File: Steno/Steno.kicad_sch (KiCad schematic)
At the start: 25 parts

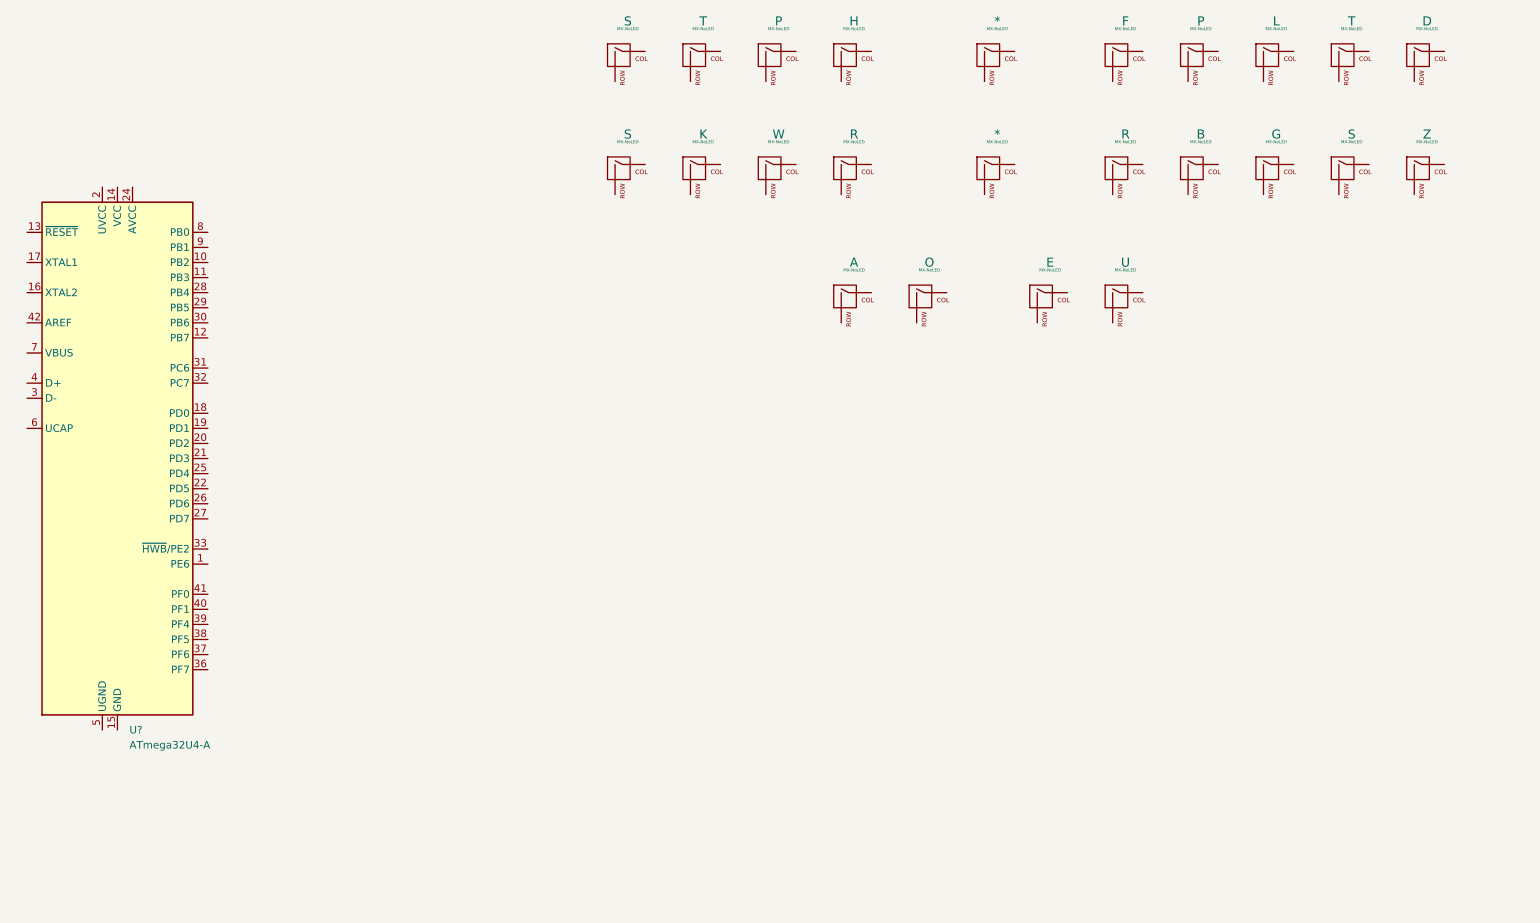
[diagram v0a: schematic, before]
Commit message: asd
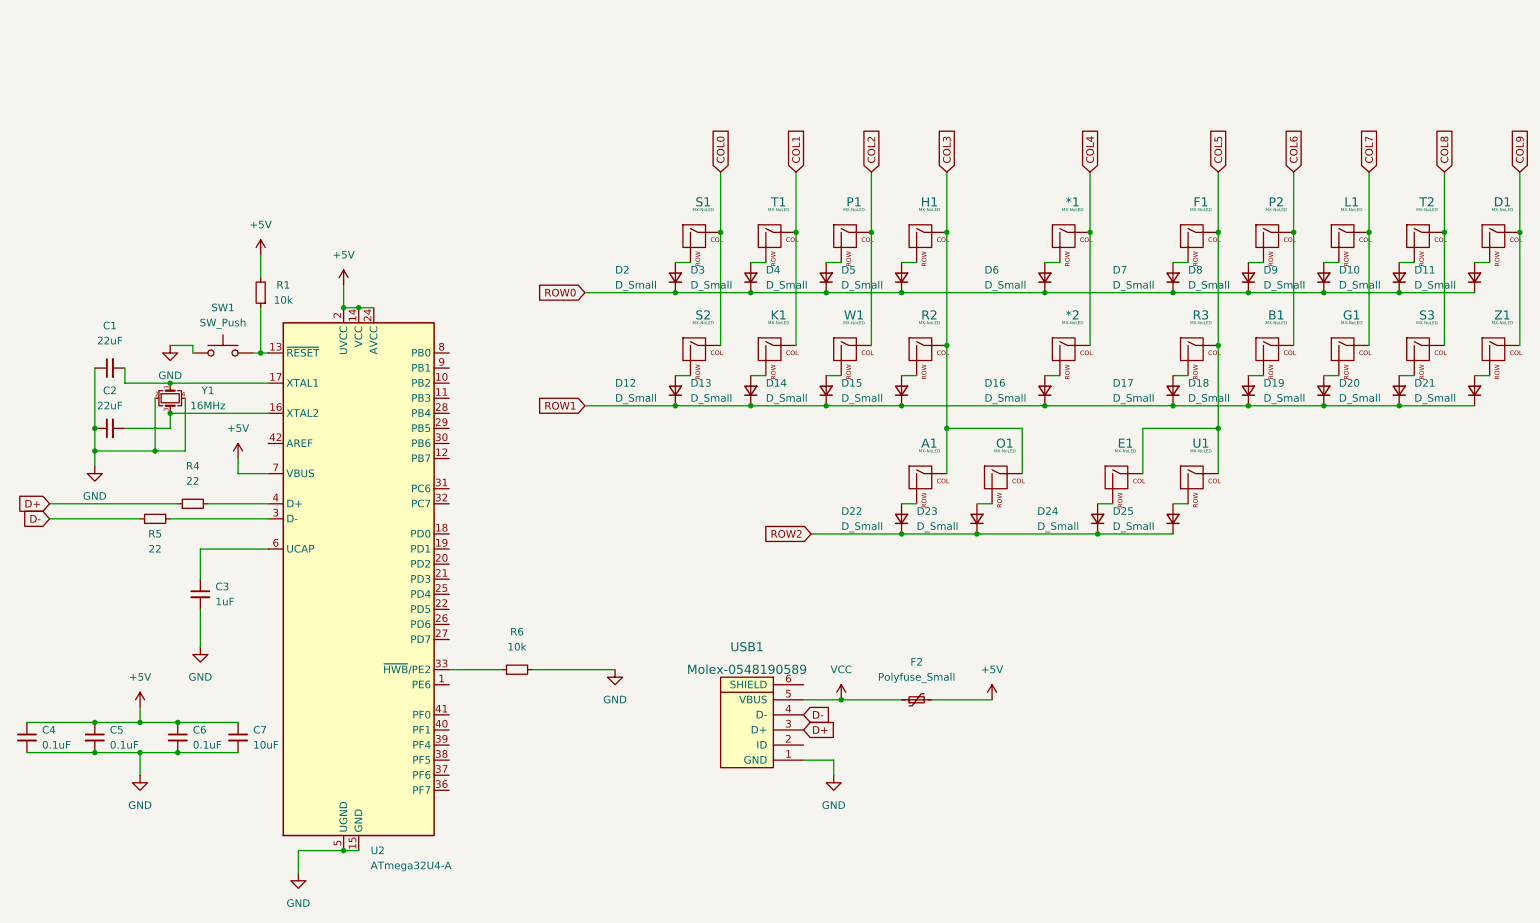
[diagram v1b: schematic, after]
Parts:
- added C1, C2: 22uF, Capacitor_SMD:C_0805_2012Metric, symbol Device:C_Small
- added C3: 1uF, Capacitor_SMD:C_0805_2012Metric, symbol Device:C_Small
- added C4, C5, C6: 0.1uF, Capacitor_SMD:C_0805_2012Metric, symbol Device:C_Small
- added C7: 10uF, Capacitor_SMD:C_0805_2012Metric, symbol Device:C_Small
- added D10, D11, D12, D13, D14, D15, D16, D17, D18, D19, D2, D20, D21, D22, D23, D24, D25, D3, D4, D5, D6, D7, D8, D9: D_Small, Diode_SMD:D_SOD-123, symbol Device:D_Small
- added F2: Polyfuse_Small, Fuse:Fuse_1206_3216Metric, symbol Device:Polyfuse_Small
- added R1, R6: 10k, Resistor_SMD:R_0805_2012Metric, symbol Device:R_Small
- added R4, R5: 22, Resistor_SMD:R_0805_2012Metric, symbol Device:R_Small
- added SW1: SW_Push, random-keyboard-parts:SKQG-1155865, symbol Switch:SW_Push
- added USB1: Molex-0548190589, random-keyboard-parts:Molex-0548190589, symbol random-keyboard-parts:Molex-0548190589
- added Y1: 16MHz, Crystal:Crystal_SMD_3225-4Pin_3.2x2.5mm, symbol Device:Crystal_GND24_Small
- *1, *2: renamed from *; footprint (none) -> MX_Alps_Hybrid:MX-1U
- A1: renamed from A; footprint (none) -> MX_Alps_Hybrid:MX-1U
- B1: renamed from B; footprint (none) -> MX_Alps_Hybrid:MX-1U
- D1: renamed from D; footprint (none) -> MX_Alps_Hybrid:MX-1U
- E1: renamed from E; footprint (none) -> MX_Alps_Hybrid:MX-1U
- F1: renamed from F; footprint (none) -> MX_Alps_Hybrid:MX-1U
- G1: renamed from G; footprint (none) -> MX_Alps_Hybrid:MX-1U
- H1: renamed from H; footprint (none) -> MX_Alps_Hybrid:MX-1U
- K1: renamed from K; footprint (none) -> MX_Alps_Hybrid:MX-1U
- L1: renamed from L; footprint (none) -> MX_Alps_Hybrid:MX-1U
- O1: renamed from O; footprint (none) -> MX_Alps_Hybrid:MX-1U
- P1, P2: renamed from P; footprint (none) -> MX_Alps_Hybrid:MX-1U
- R2, R3: renamed from R; footprint (none) -> MX_Alps_Hybrid:MX-1U
- S1, S2, S3: renamed from S; footprint (none) -> MX_Alps_Hybrid:MX-1U
- T1, T2: renamed from T; footprint (none) -> MX_Alps_Hybrid:MX-1U
- U1: renamed from U; footprint (none) -> MX_Alps_Hybrid:MX-1U
- W1: renamed from W; footprint (none) -> MX_Alps_Hybrid:MX-1U
- Z1: renamed from Z; footprint (none) -> MX_Alps_Hybrid:MX-1U
- gave numbers to parts that had none: 1
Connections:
- net COL5: now reaches E1.1 (COL)
- net COL5: now also F1.1 (COL), R3.1 (COL), U1.1 (COL)
- net at E1.2 (ROW): now also D24.2 (A)
- net COL8: now reaches T2.1 (COL)
- net COL8: now also S3.1 (COL)
- net at T2.2 (ROW): now also D10.2 (A)
- net COL2: now reaches P1.1 (COL)
- net COL2: now also W1.1 (COL)
- net at P1.2 (ROW): now also D4.2 (A)
- net COL6: now reaches P2.1 (COL)
- net COL6: now also B1.1 (COL)
- net at P2.2 (ROW): now also D8.2 (A)
- net COL7: now reaches L1.1 (COL)
- net COL7: now also G1.1 (COL)
- net at L1.2 (ROW): now also D9.2 (A)
- net at U1.2 (ROW): now also D25.2 (A)
- net COL1: now reaches T1.1 (COL)
- net COL1: now also K1.1 (COL)
- net at T1.2 (ROW): now also D3.2 (A)
- net COL9: now reaches Z1.1 (COL)
- net COL9: now also D1.1 (COL)
- net at Z1.2 (ROW): now also D21.2 (A)
- net COL3: now reaches O1.1 (COL)
- net COL3: now also A1.1 (COL), H1.1 (COL), R2.1 (COL)
- net at O1.2 (ROW): now also D23.2 (A)
- net at H1.2 (ROW): now also D5.2 (A)
- net at A1.2 (ROW): now also D22.2 (A)
- net COL0: now reaches S1.1 (COL)
- net COL0: now also S2.1 (COL)
- net at S1.2 (ROW): now also D2.2 (A)
- net at F1.2 (ROW): now also D7.2 (A)
- net at S2.2 (ROW): now also D12.2 (A)
- net at D1.2 (ROW): now also D11.2 (A)
- net at B1.2 (ROW): now also D18.2 (A)
- net at R2.2 (ROW): now also D15.2 (A)
- net COL4: now reaches *1.1 (COL)
- net COL4: now also *2.1 (COL)
- net at *1.2 (ROW): now also D6.2 (A)
- net at U2.13 (~{RESET}): now also R1.1, SW1.2
- net +5V: now reaches U2.14 (VCC), U2.34 (VCC)
- net +5V: now also U2.2 (UVCC), U2.24 (AVCC), U2.44 (AVCC), U2.7 (VBUS), C4.1, C5.1, C6.1, C7.1, F2.2, R1.2
- net GND: now reaches U2.15 (GND), U2.23 (GND), U2.35 (GND), U2.43 (GND)
- net GND: now also U2.5 (UGND), C1.1, C2.1, C3.2, C4.2, C5.2, C6.2, C7.2, R6.2, SW1.1, USB1.1 (GND), Y1.2, Y1.4
- net at U2.16 (XTAL2): now also C2.2, Y1.3
- net at U2.17 (XTAL1): now also C1.2, Y1.1
- net at U2.3 (D-): now also R5.2
- net at U2.33 (~{HWB}/PE2): now also R6.1
- net at U2.4 (D+): now also R4.2
- net at U2.6 (UCAP): now also C3.1
- net at G1.2 (ROW): now also D19.2 (A)
- net at K1.2 (ROW): now also D13.2 (A)
- net at R3.2 (ROW): now also D17.2 (A)
- net at W1.2 (ROW): now also D14.2 (A)
- net at *2.2 (ROW): now also D16.2 (A)
- net at S3.2 (ROW): now also D20.2 (A)
- new net D+: R4.1, USB1.3 (D+)
- new net D-: R5.1, USB1.4 (D-)
- new net ROW0: D10.1 (K), D11.1 (K), D2.1 (K), D3.1 (K), D4.1 (K), D5.1 (K), D6.1 (K), D7.1 (K), D8.1 (K), D9.1 (K)
- new net ROW1: D12.1 (K), D13.1 (K), D14.1 (K), D15.1 (K), D16.1 (K), D17.1 (K), D18.1 (K), D19.1 (K), D20.1 (K), D21.1 (K)
- new net ROW2: D22.1 (K), D23.1 (K), D24.1 (K), D25.1 (K)
- new net VCC: F2.1, USB1.5 (VBUS)
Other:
- moved on the sheet: *1, *2, A1, B1, D1, E1, F1, G1, H1, K1, L1, O1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
